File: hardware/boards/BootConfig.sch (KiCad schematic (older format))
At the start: 13 parts, among them J3 Conn_02x05_Odd_Even, SW1 SW_DIP_x03, U1 ECP5UM5G-381caBGA, U3 CYUSB3014, U5 128MiB

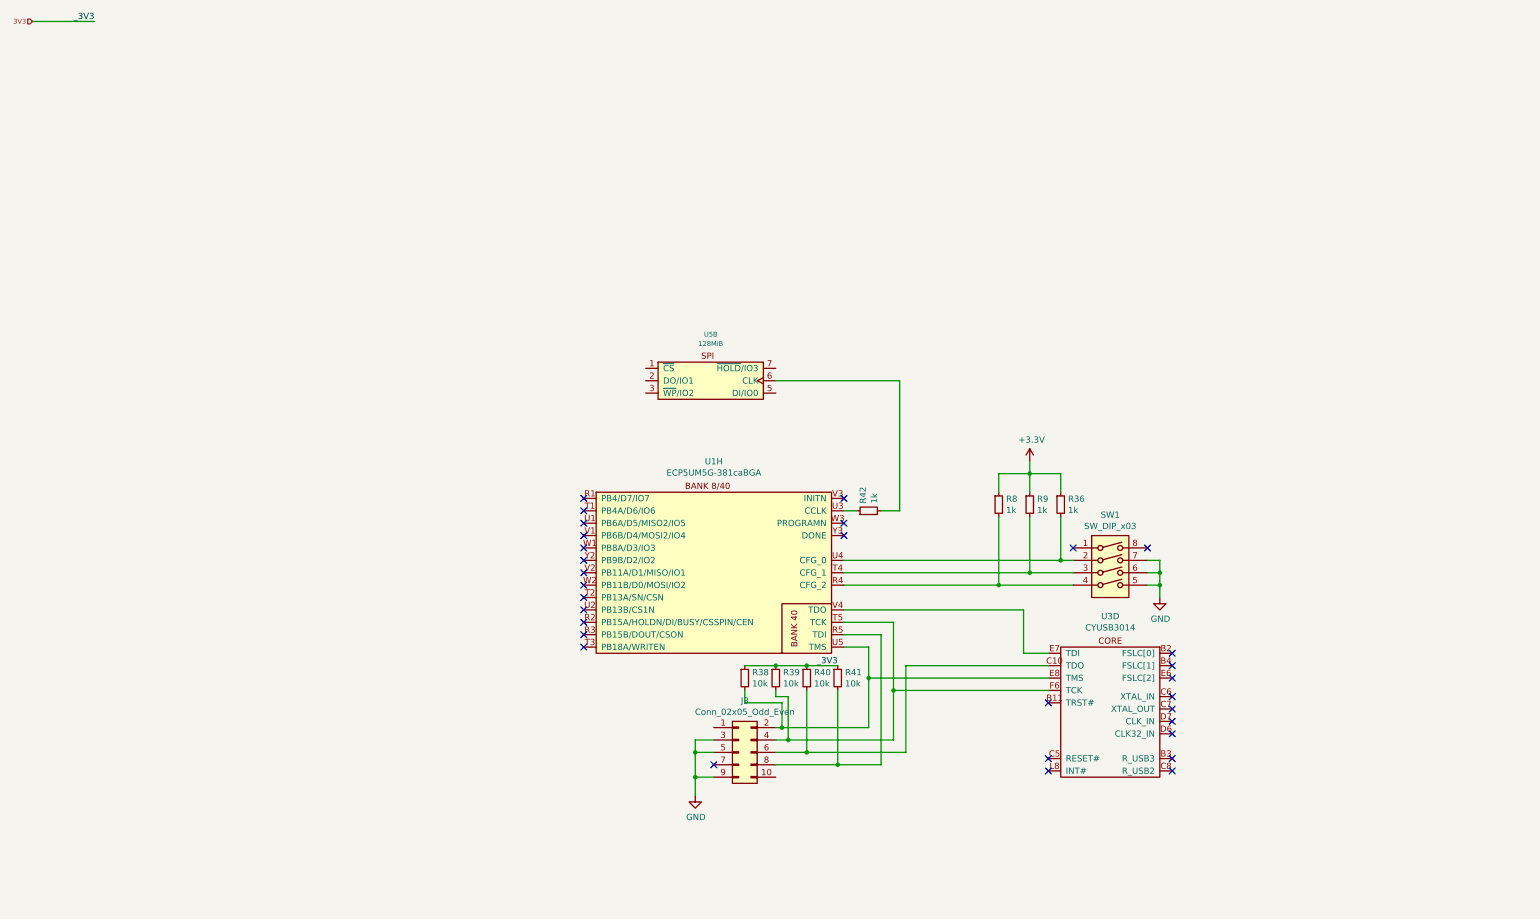
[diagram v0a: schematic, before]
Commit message: Added a bunch of stuff having to do with JTAG and the FPGA flash / bring up
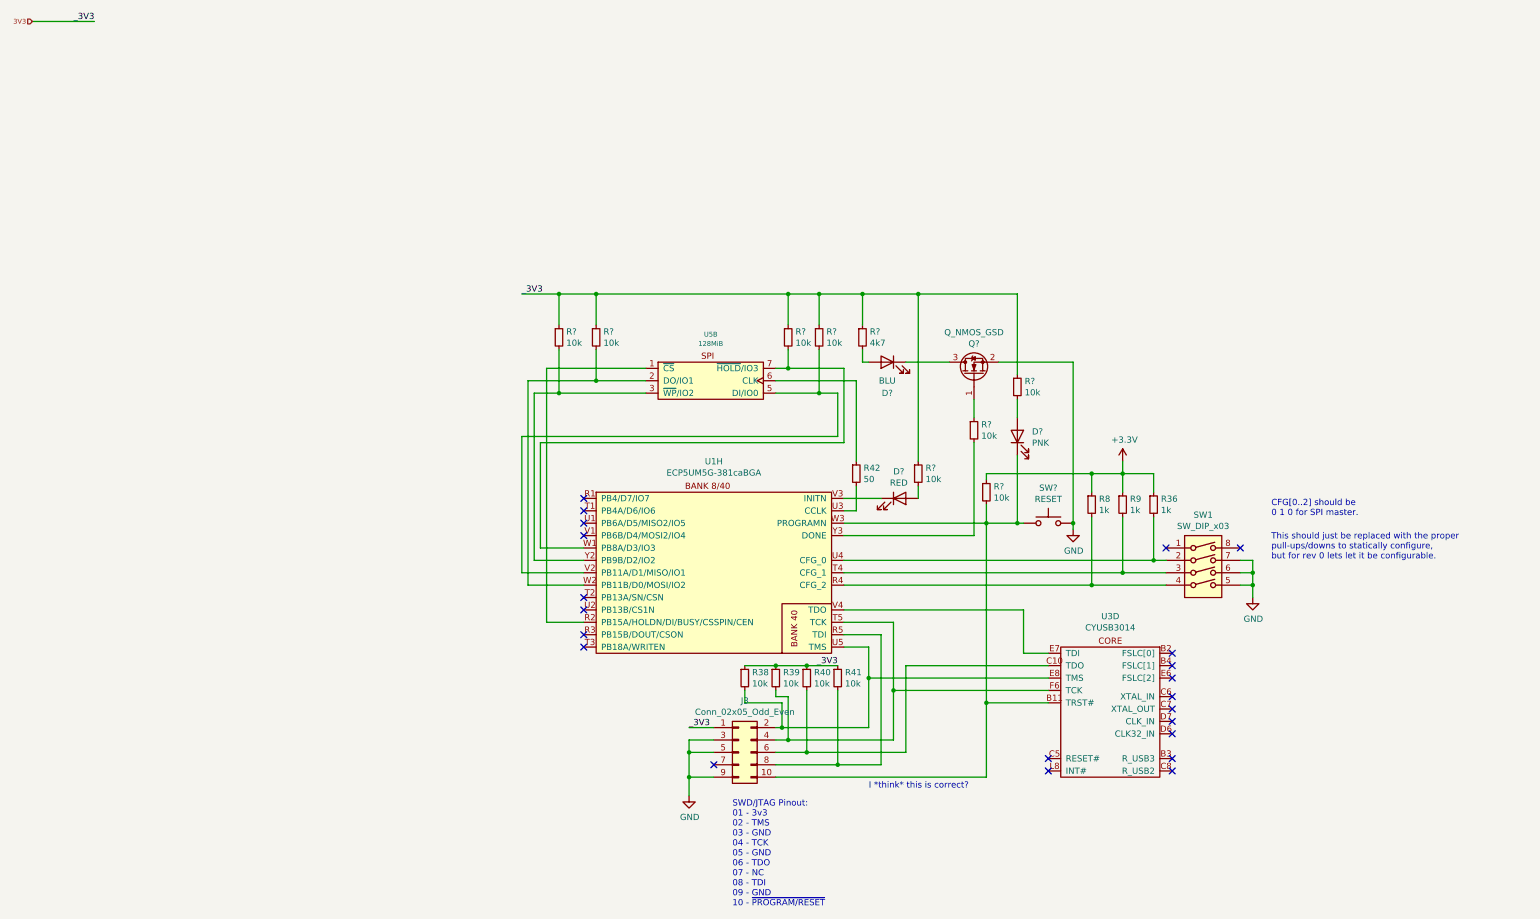
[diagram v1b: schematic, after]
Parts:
- added D?: PNK, LED_SMD:LED_0603_1608Metric, symbol Device:LED
- added D?: RED, LED_SMD:LED_0603_1608Metric, symbol Device:LED
- added D?: BLU, LED_SMD:LED_0603_1608Metric, symbol Device:LED
- added Q?: Q_NMOS_GSD, Package_TO_SOT_SMD:SOT-23, symbol Device:Q_NMOS_GSD
- added R? (x8): 10k, Resistor_SMD:R_0603_1608Metric, symbol Device:R_Small
- added R?: 4k7, Resistor_SMD:R_0603_1608Metric, symbol Device:R_Small
- added SW?: RESET, symbol Switch:SW_Push
- R42: value 1k -> 50; MPN CRCW06031K00FKEAHP -> CRCW060350R0FKEA
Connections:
- net +3V3: now also R?.1
- net 3V3: now also J3.1 (Pin_1), R?.1, R?.1, R?.1, R?.1, R?.1, R?.1, R?.1
- net GND: now also Q?.2 (S), SW?.2
- net at U5.1 (~CS): now also U1.R2 (PB15A/HOLDN/DI/BUSY/CSSPIN/CEN)
- net at U5.2 (DO/IO1): now also U1.W2 (PB11B/D0/MOSI/IO2), R?.2
- net at U5.3 (~WP~/IO2): now also U1.Y2 (PB9B/D2/IO2), R?.2
- net at U5.5 (DI/IO0): now also U1.V2 (PB11A/D1/MISO/IO1), R?.2
- net at U5.6 (CLK): now also R42.1; no longer R42.2
- net at U5.7 (~HOLD~/IO3): now also U1.W1 (PB8A/D3/IO3), R?.2
- net at U1.U3 (CCLK): now also R42.2; no longer R42.1
- net at U1.V3 (INITN): now also D?.1 (K)
- net at U1.W3 (PROGRAMN): now also J3.10 (Pin_10), U3.B11 (TRST#), D?.1 (K), R?.2, SW?.1
- net at U1.Y3 (DONE): now also R?.2
- new net: D?.2 (A), R?.2 (x3)
- new net: Q?.1 (G), R?.1
- new net: D?.1 (K), Q?.3 (D)
- no-connect marks 31 -> 22
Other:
- note added: "CFG[0..2] should be\n0 1 0 for SPI master."
- note added: "I *think* this is correct?"
- note added: "SWD/JTAG Pinout:\n01 - 3v3\n02 - TMS\n03 - GND\n04 - TCK\n05 - GND\n06 - TDO\n07 - NC\n08 - TDI\n09 - GND\n10 - ~PROGRAM/RESET"
- note added: "This should just be replaced with the proper\npull-ups/downs to statically configure,\nbut for rev 0 lets let it be configurable."
- moved on the sheet: R36, R42, R8, R9, SW1
